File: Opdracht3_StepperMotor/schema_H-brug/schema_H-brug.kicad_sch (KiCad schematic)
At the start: 31 parts, among them J1 Conn_01x04, M1 Motor_DC, Q1 Q_PMOS_GDS, Q2 Q_NMOS_GDS, Q3 Q_PMOS_GDS, Q4 Q_NMOS_GDS

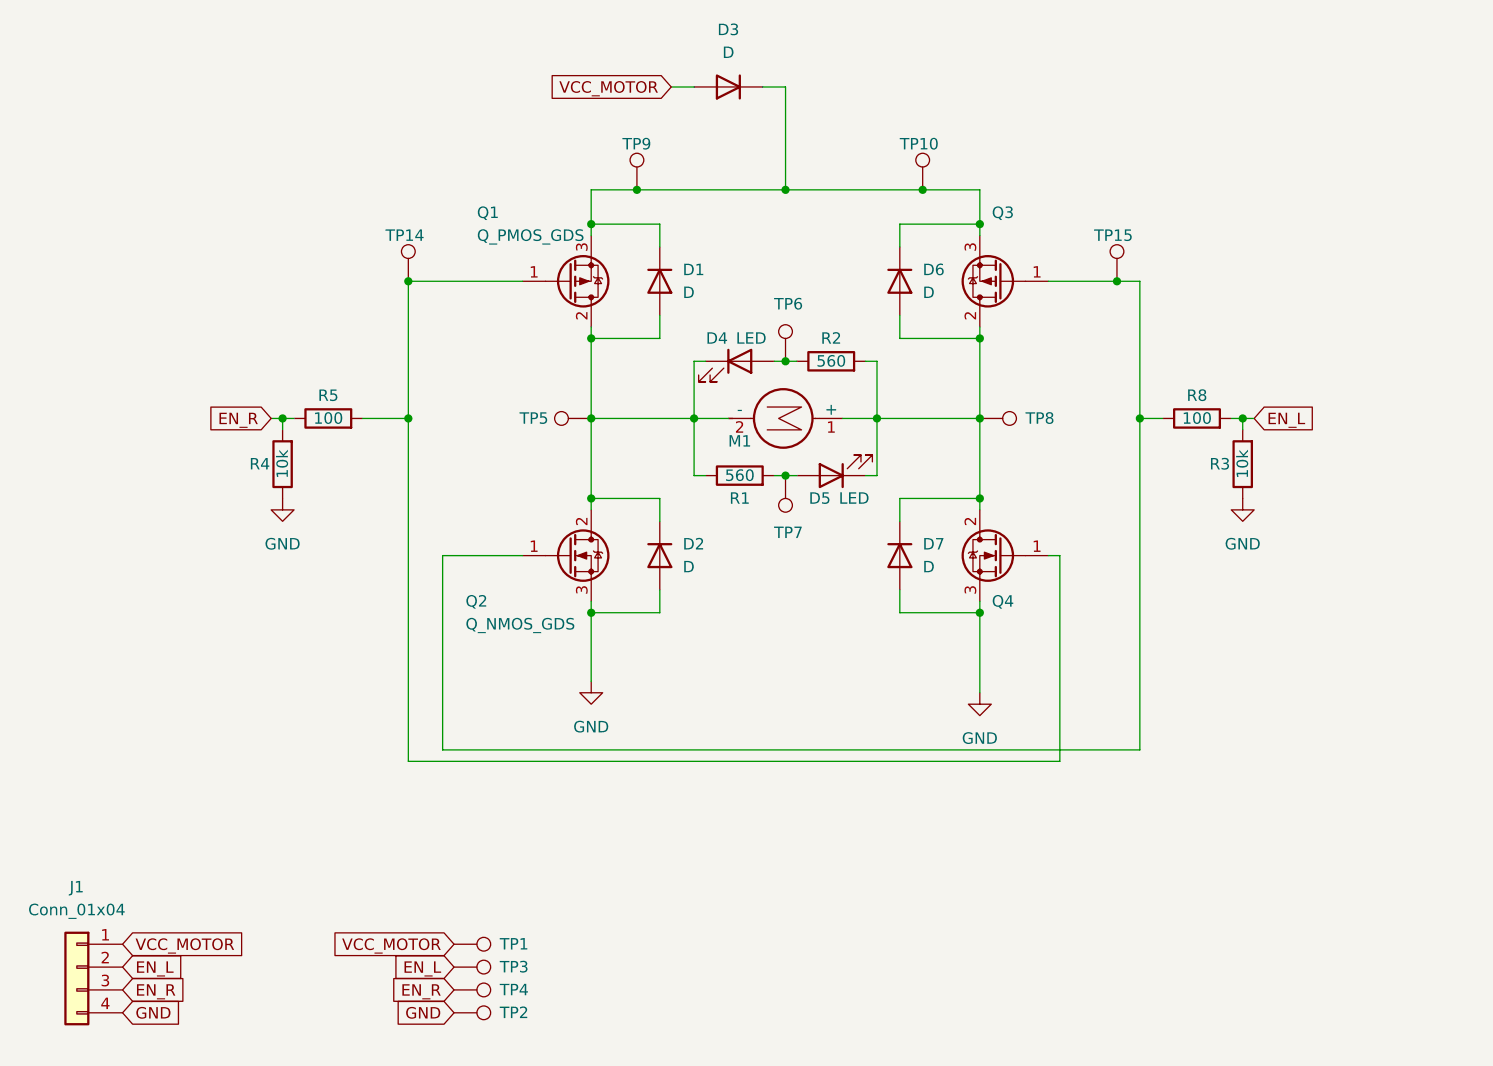
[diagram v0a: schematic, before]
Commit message: update schema
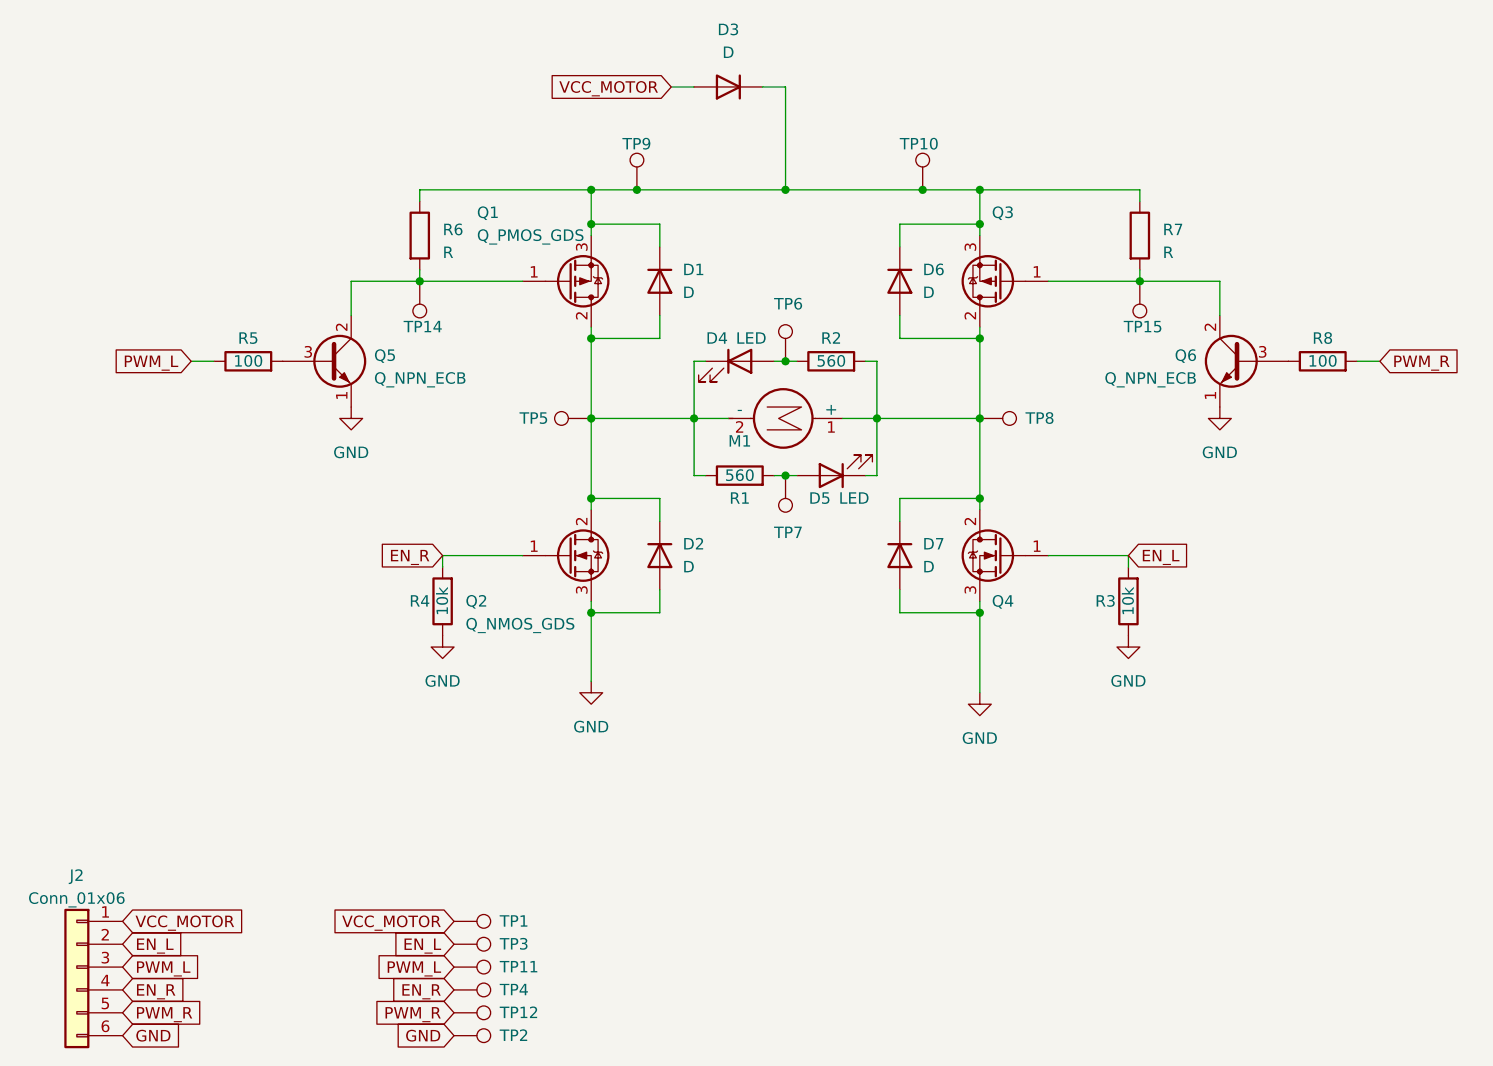
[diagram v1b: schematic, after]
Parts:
- removed J1: Conn_01x04, Connector_PinHeader_2.54mm:PinHeader_1x04_P2.54mm_Vertical, symbol Connector_Generic:Conn_01x04
- added J2: Conn_01x06, symbol Connector_Generic:Conn_01x06
- added Q5, Q6: Q_NPN_ECB, symbol Device:Q_NPN_ECB
- added R6, R7: R, symbol Device:R
- added TP11, TP12: TestPoint, TestPoint:TestPoint_Keystone_5005-5009_Compact, symbol Connector:TestPoint
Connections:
- net EN_L: now also Q4.1 (G), J2.2 (Pin_2); no longer R8.2
- net EN_R: now also Q2.1 (G), J2.4 (Pin_4); no longer R5.1
- net GND: now also J2.6 (Pin_6), Q5.1 (E), Q6.1 (E)
- net VCC_MOTOR: now also J2.1 (Pin_1)
- net at D1.1 (K), D3.1 (K), D6.1 (K)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: now also R6.1, R7.1
- net at Q3.1 (G), TP15.1: now also Q6.2 (C), R7.2; no longer Q2.1 (G), R8.1
- net at Q1.1 (G), TP14.1: now also Q5.2 (C), R6.2; no longer Q4.1 (G), R5.2
- new net: Q5.3 (B), R5.2
- new net: Q6.3 (B), R8.1
- new net PWM_L: J2.3 (Pin_3), R5.1, TP11.1
- new net PWM_R: J2.5 (Pin_5), R8.2, TP12.1
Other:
- moved on the sheet: R3, R4, R5, R8, TP1, TP14, TP15, TP2, TP3
